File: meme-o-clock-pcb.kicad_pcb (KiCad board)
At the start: 4 copper layers, 88 x 100 mm, 24 parts, among them J1 USB_C_Receptacle_USB2.0_16P, J2 Conn_01x04_Pin, J3 Conn_01x02_Pin, J4 Conn_01x03_Pin, SW1 SW_Push, SW2 SW_Push, SW3 SW_Push, SW4 SW_Push, U1 MAX98357A, U2 APDS-9306

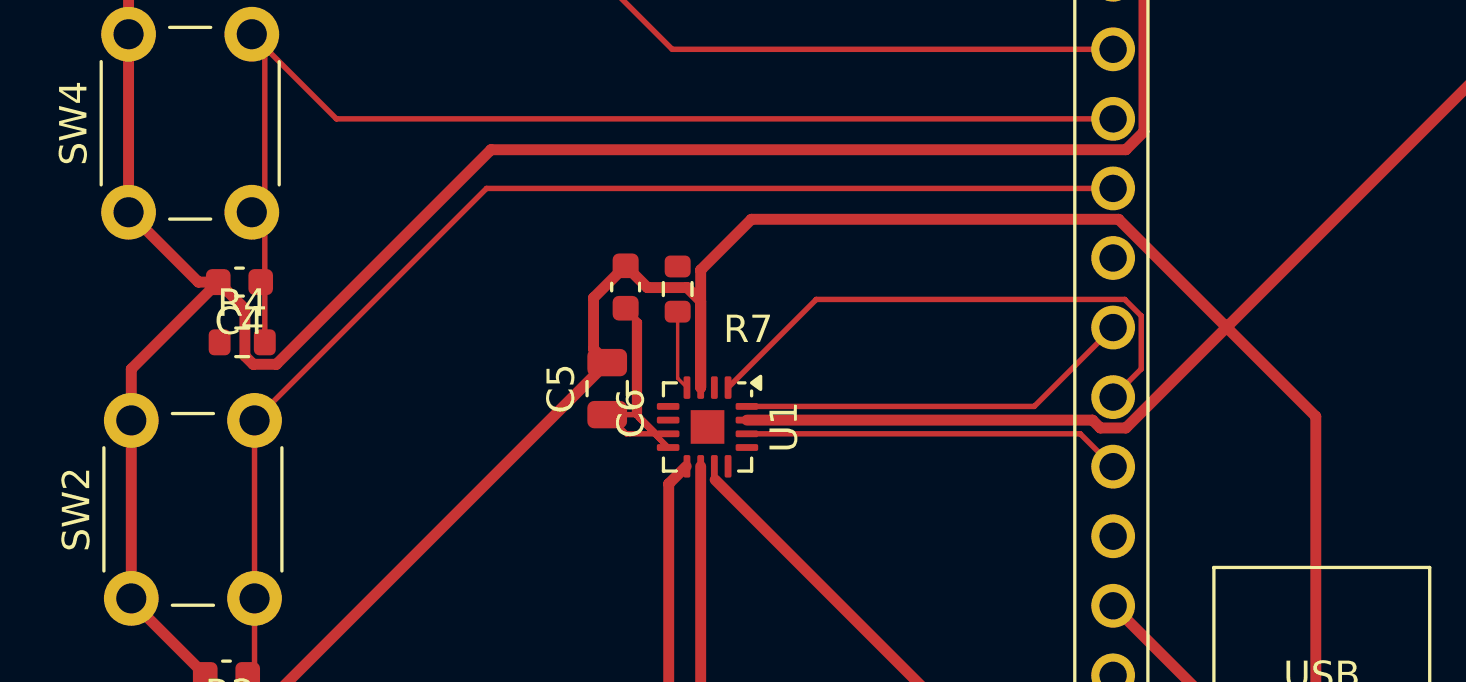
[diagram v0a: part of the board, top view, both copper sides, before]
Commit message: Autosave
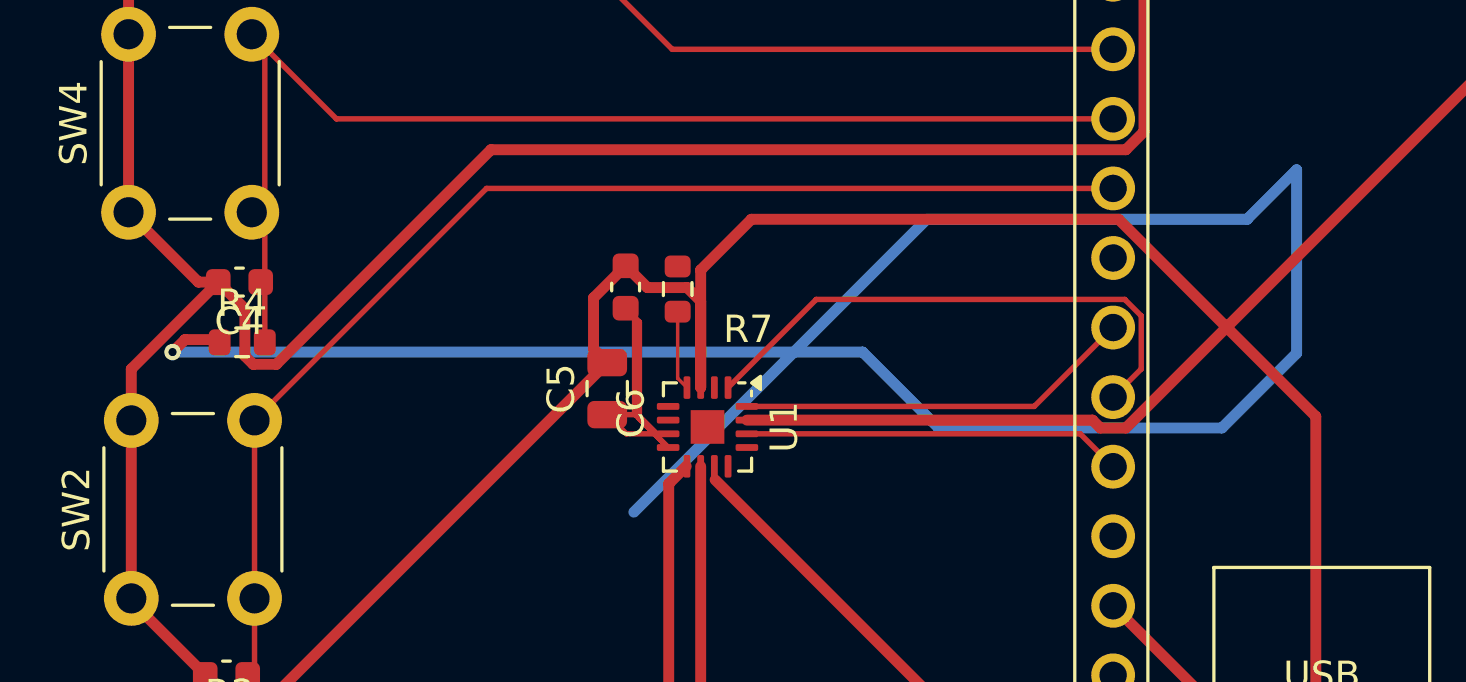
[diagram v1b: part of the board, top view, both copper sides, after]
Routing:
- net +3V3: track 0.25 -> 81.6 mm, vias 0 -> 1
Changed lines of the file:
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@@
+	)
+	(segment
+		(start 79.611712 99.3)
+		(end 79.155856 99.755856)
+		(width 0.4)
+		(layer "F.Cu")
+		(net "+3V3")
+	)
+	(segment
+		(start 80.8 99.4)
+		(end 80.7 99.3)
+		(width 0.4)
+		(layer "F.Cu")
+		(net "+3V3")
+	)
+	(segment
+		(start 80.875 99.4)
+		(end 80.8 99.4)
+		(width 0.4)
+		(layer "F.Cu")
+		(net "+3V3")
+	)
+	(segment
+		(start 80.7 99.3)
+		(end 79.611712 99.3)
+		(width 0.4)
+		(layer "F.Cu")
+		(net "+3V3")
+	)
+	(via
+		(at 79.155856 99.755856)
+		(size 0.6)
+		(drill 0.3)
+		(layers "F.Cu" "B.Cu")
+		(net "+3V3")
+	)
+	(segment
+		(start 104.355856 99.755856)
+		(end 107.127 102.527)
+		(width 0.4)
+		(layer "B.Cu")
+		(net "+3V3")
+	)
+	(segment
+		(start 79.155856 99.755856)
+		(end 104.355856 99.755856)
+		(width 0.4)
+		(layer "B.Cu")
+		(net "+3V3")
+	)
+	(segment
+		(start 120.2 99.8)
+		(end 120.2 93.1)
+		(width 0.4)
+		(layer "B.Cu")
+		(net "+3V3")
+	)
+	(segment
+		(start 120.2 93.1)
+		(end 118.393 94.907)
+		(width 0.4)
+		(layer "B.Cu")
+		(net "+3V3")
+	)
+	(segment
+		(start 118.393 94.907)
+		(end 106.693 94.907)
+		(width 0.4)
+		(layer "B.Cu")
+		(net "+3V3")
+	)
+	(segment
+		(start 106.693 94.907)
+		(end 96 105.6)
+		(width 0.4)
+		(layer "B.Cu")
+		(net "+3V3")
+	)
+	(segment
+		(start 107.127 102.527)
+		(end 117.473 102.527)
+		(width 0.4)
+		(layer "B.Cu")
+		(net "+3V3")
+	)
+	(segment
+		(start 117.473 102.527)
+		(end 120.2 99.8)
+		(width 0.4)
+		(layer "B.Cu")
+		(net "+3V3")
 	)
 	(segment
